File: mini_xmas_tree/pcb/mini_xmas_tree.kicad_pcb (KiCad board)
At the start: 2 copper layers, 19 parts, among them J1 Conn_01x02, J2 Conn_01x02, J3 Conn_01x02, J4 Conn_01x02, Q1 BC817, Q2 BC817, Q3 BC817, Q4 BC817

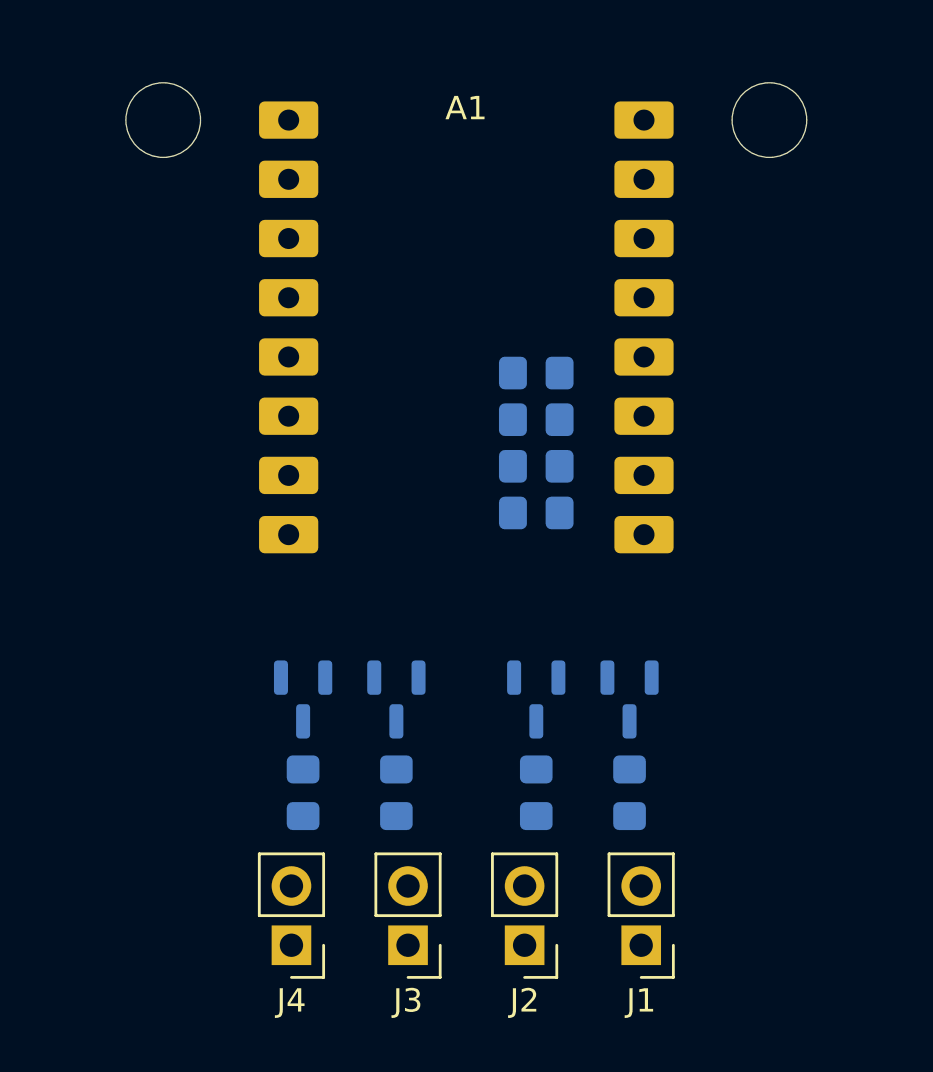
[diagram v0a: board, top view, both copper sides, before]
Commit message: create gcode
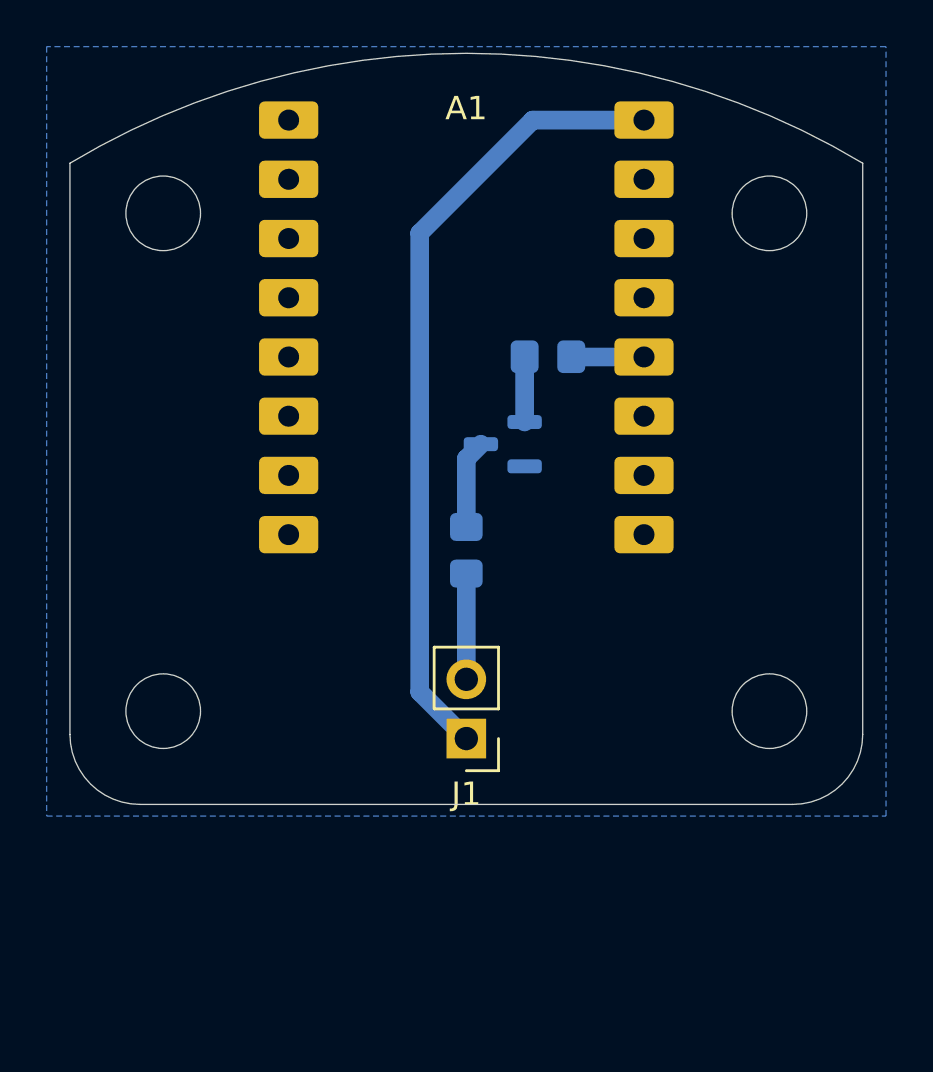
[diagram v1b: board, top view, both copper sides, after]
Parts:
- removed J2, J3, J4: Conn_01x02, Connector_PinHeader_2.54mm:PinHeader_1x02_P2.54mm_Vertical
- removed Q2, Q3, Q4: BC817, Package_TO_SOT_SMD:SOT-23
- removed R3, R4, R5, R6, R7, R8: R, Resistor_SMD:R_0805_2012Metric_Pad1.20x1.40mm_HandSolder
- added H3: MountingHole, MountingHole:MountingHole_3.2mm_M3, F.Cu at (127.0, 95.5)
- added H4: MountingHole, MountingHole:MountingHole_3.2mm_M3, F.Cu at (153.0, 95.5)
- moved R2 12.5 mm to (140.0, 88.6)
- moved Q1 12.2 mm to (141.6, 84.0), turned to 180 degrees
- moved J1 11.6 mm to (140.0, 96.7)
- moved H1 4.00 mm to (127.0, 74.2)
- moved H2 4.00 mm to (153.0, 74.2)
- moved R1 0.86 mm to (143.5, 80.3)
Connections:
- net /LED_STRING_3 renamed /LED_STRING_CTRL
- A1 pad 10: /LED_STRING_1 -> unconnected-(A1-GPIO01-Pad10)
- A1 pad 11: /LED_STRING_2 -> unconnected-(A1-GPIO02-Pad11)
- A1 pad 9: /LED_STRING_0 -> unconnected-(A1-GPIO00-Pad9)
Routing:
- net +5V: track 0.00 -> 34.1 mm
- net Net-(J1-Pin_2): track 0.00 -> 4.54 mm
- net Net-(Q1-C): track 0.00 -> 3.81 mm
- net /LED_STRING_CTRL: track 0.00 -> 3.12 mm
- net Net-(Q1-B): track 0.00 -> 2.80 mm
- added copper zone on B.Cu, net GND
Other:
- board outline added: 34 x 32.2 mm
